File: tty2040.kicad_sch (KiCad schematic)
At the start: 16 parts, among them U13 YC162-FR-072K4L, U14 YC162-FR-072K4L, U15 YC162-FR-072K4L

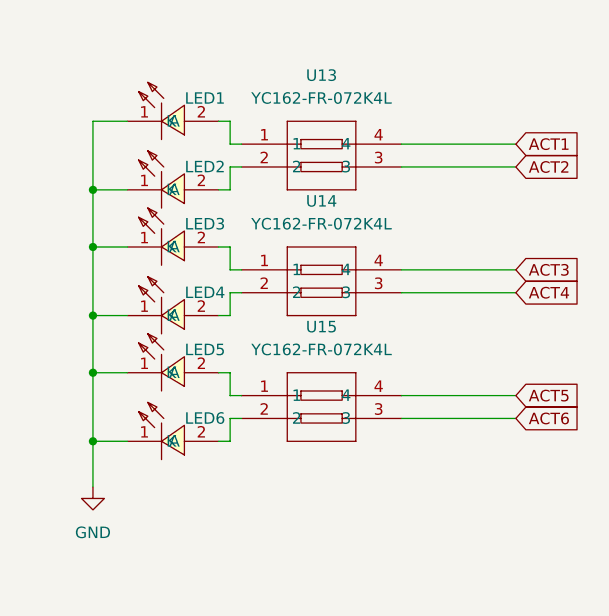
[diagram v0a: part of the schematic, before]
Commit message: Rev b begin
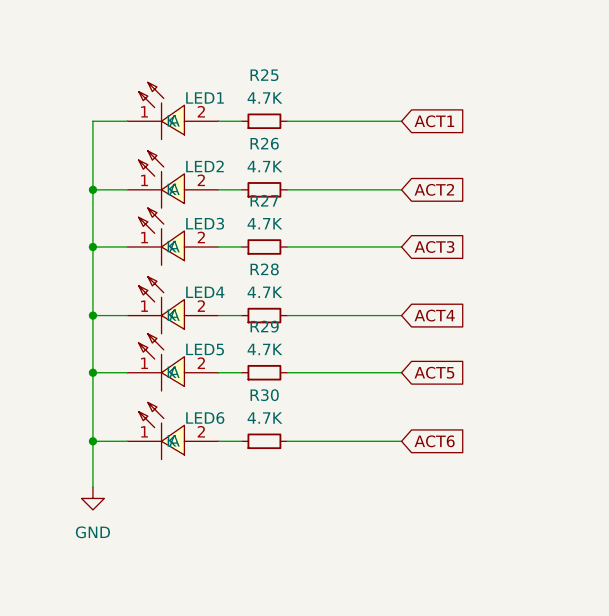
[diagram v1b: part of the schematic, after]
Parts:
- removed U13, U14, U15: YC162-FR-072K4L, local:RES-ARRAY-SMD_0603-4P-L1.6-W1.6-BL, symbol local:YC162-FR-072K4L
- added R25, R26, R27, R28, R29, R30: 4.7K, Resistor_SMD:R_0805_2012Metric, symbol Device:R_Small
- LED1, LED2, LED3, LED4, LED5, LED6: footprint local:LED0603-RD -> Diode_SMD:D_0805_2012Metric; LCSC C2286 -> C2297; LCSC Part C2286 -> C2297
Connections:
- net ACT1: now also R25.2
- net ACT2: now also R26.2
- net ACT3: now also R27.2
- net ACT4: now also R28.2
- net ACT5: now also R29.2
- net ACT6: now also R30.2
- net at LED2.2 (A): now also R26.1
- net at LED5.2 (A): now also R29.1
- net at LED6.2 (A): now also R30.1
- net at LED3.2 (A): now also R27.1
- net at LED4.2 (A): now also R28.1
- net at LED1.2 (A): now also R25.1

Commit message: revB continue routing
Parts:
- A1: footprint Module_RaspberryPi_Pico:RaspberryPi_Pico_Common -> Module_RaspberryPi_Pico:RaspberryPi_Pico_Original_SMD_HandSolder
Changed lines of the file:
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@@
 			)
 		)
-		(property "Footprint" "Module_RaspberryPi_Pico:RaspberryPi_Pico_Common"
+		(property "Footprint" "Module_RaspberryPi_Pico:RaspberryPi_Pico_Original_SMD_HandSolder"
 			(at 99.06 149.86 0)
 			(effects
